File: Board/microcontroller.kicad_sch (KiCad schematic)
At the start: 31 parts, among them J10 FAN, J11 DUO LED, J9 ICSP, Q7 IRLML2502, SW1 CALIBRATE, U2 PIC18F2480-ISO, Y1 10 MHz

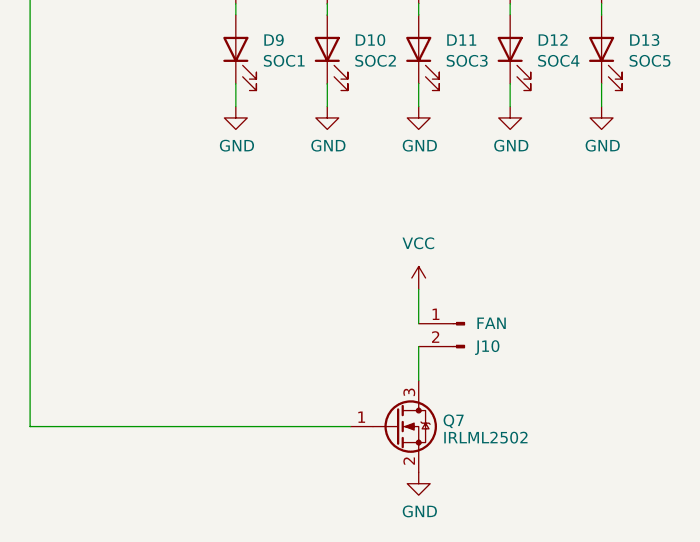
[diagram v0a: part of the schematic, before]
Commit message: New layout
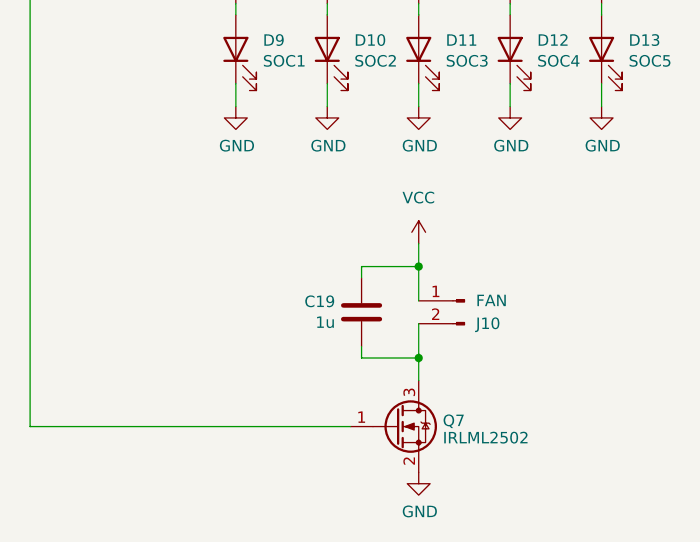
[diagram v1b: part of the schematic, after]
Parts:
- added C19: 1u, Capacitor_SMD:C_1206_3216Metric, symbol Device:C
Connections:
- net VCC: now also C19.1
- net at J10.2 (Pin_2), Q7.3 (D): now also C19.2
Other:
- moved on the sheet: J10
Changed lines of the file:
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@@
 	)
 	(junction
+		(at 231.14 142.24)
+		(diameter 0)
+		(color 0 0 0 0)
+	)
+	(junction
 		(at 217.17 57.15)
 		(diameter 0)
@@
 	)
 	(junction
+		(at 231.14 132.08)
+		(diameter 0)
+		(color 0 0 0 0)
+	)
+	(junction
 		(at 118.11 48.26)
 		(diameter 0)
@@
 	(wire
 		(pts
-			(xy 231.14 140.97) (xy 231.14 144.78)
+			(xy 231.14 138.43) (xy 231.14 142.24)
 		)
 		(stroke
@@
 	(wire
 		(pts
-			(xy 231.14 134.62) (xy 231.14 138.43)
+			(xy 231.14 129.54) (xy 231.14 132.08)
 		)
 		(stroke
@@
 	(wire
 		(pts
+			(xy 224.79 142.24) (xy 231.14 142.24)
+		)
+		(stroke
+			(width 0)
+			(type default)
+		)
+	)
+	(wire
+		(pts
 			(xy 168.91 120.65) (xy 149.86 120.65)
 		)
@@
 	(wire
 		(pts
+			(xy 224.79 133.35) (xy 224.79 132.08)
+		)
+		(stroke
+			(width 0)
+			(type default)
+		)
+	)
+	(wire
+		(pts
 			(xy 217.17 57.15) (xy 217.17 76.2)
 		)
@@
 	(wire
 		(pts
+			(xy 231.14 132.08) (xy 231.14 135.89)
+		)
+		(stroke
+			(width 0)
+			(type default)
+		)
+	)
+	(wire
+		(pts
 			(xy 220.98 114.3) (xy 220.98 111.76)
 		)
@@
 	(wire
 		(pts
+			(xy 224.79 132.08) (xy 231.14 132.08)
+		)
+		(stroke
+			(width 0)
+			(type default)
+		)
+	)
+	(wire
+		(pts
 			(xy 31.75 54.61) (xy 34.29 54.61)
 		)
@@
 	(wire
 		(pts
+			(xy 224.79 140.97) (xy 224.79 142.24)
+		)
+		(stroke
+			(width 0)
+			(type default)
+		)
+	)
+	(wire
+		(pts
 			(xy 148.59 73.66) (xy 201.93 73.66)
 		)
@@
 	(wire
 		(pts
+			(xy 231.14 142.24) (xy 231.14 144.78)
+		)
+		(stroke
+			(width 0)
+			(type default)
+		)
+	)
+	(wire
+		(pts
 			(xy 36.83 50.8) (xy 36.83 52.07)
 		)
@@
 	)
 	(symbol
+		(lib_id "Device:C")
+		(at 224.79 137.16 0)
+		(mirror y)
+		(unit 1)
+		(exclude_from_sim no)
+		(in_bom yes)
+		(on_board yes)
+		(dnp no)
+		(property "Reference" "C19"
+			(at 221.869 135.9916 0)
+			(effects
+				(font
+					(size 1.27 1.27)
+				)
+				(justify left)
+			)
+		)
+		(property "Value" "1u"
+			(at 221.869 138.303 0)
+			(effects
+				(font
+					(size 1.27 1.27)
+				)
+				(justify left)
+			)
+		)
+		(property "Footprint" "Capacitor_SMD:C_1206_3216Metric"
+			(at 223.8248 140.97 0)
+			(effects
+				(font
+					(size 1.27 1.27)
+				)
+				(hide yes)
+			)
+		)
+		(property "Datasheet" "~"
+			(at 224.79 137.16 0)
+			(effects
+				(font
+					(size 1.27 1.27)
+				)
+				(hide yes)
+			)
+		)
+		(property "Description" ""
+			(at 224.79 137.16 0)
+			(effects
+				(font
+					(size 1.27 1.27)
+				)
+				(hide yes)
+			)
+		)
+		(pin "1"
+		)
+		(pin "2"
+		)
+		(instances
+			(project "12VSupport"
+				(path "/f0c44745-560b-4dea-806a-2541c74a511b/3945f109-57ed-41f6-8253-6d6ba9eb298d"
+					(reference "C19")
+					(unit 1)
+				)
+			)
+		)
+	)
+	(symbol
 		(lib_id "power:GND")
 		(at 41.91 101.6 0)
@@
 	(symbol
 		(lib_id "Connector:Conn_01x02_Pin")
-		(at 236.22 138.43 0)
+		(at 236.22 135.89 0)
 		(mirror y)
 		(unit 1)
@@
 		(dnp no)
 		(property "Reference" "J10"
-			(at 237.49 140.9701 0)
+			(at 237.49 138.4301 0)
 			(effects
 				(font
@@
 		)
 		(property "Value" "FAN"
-			(at 237.49 138.4301 0)
+			(at 237.49 135.8901 0)
 			(effects
 				(font
@@
 		)
 		(property "Footprint" "Connector_JST:JST_XH_B2B-XH-A_1x02_P2.50mm_Vertical"
-			(at 236.22 138.43 0)
+			(at 236.22 135.89 0)
 			(effects
 				(font
@@
 		)
 		(property "Datasheet" "~"
-			(at 236.22 138.43 0)
+			(at 236.22 135.89 0)
 			(effects
 				(font
@@
 		)
 		(property "Description" "Generic connector, single row, 01x02, script generated"
-			(at 236.22 138.43 0)
+			(at 236.22 135.89 0)
 			(effects
 				(font
@@
 	(symbol
 		(lib_id "power:VCC")
-		(at 231.14 134.62 0)
+		(at 231.14 129.54 0)
 		(unit 1)
 		(exclude_from_sim no)
@@
 		(fields_autoplaced yes)
 		(property "Reference" "#PWR040"
-			(at 231.14 138.43 0)
+			(at 231.14 133.35 0)
 			(effects
 				(font
@@
 		)
 		(property "Value" "VCC"
-			(at 231.14 129.54 0)
+			(at 231.14 124.46 0)
 			(effects
 				(font
@@
 		)
 		(property "Footprint" ""
-			(at 231.14 134.62 0)
+			(at 231.14 129.54 0)
 			(effects
 				(font
@@
 		)
 		(property "Datasheet" ""
-			(at 231.14 134.62 0)
+			(at 231.14 129.54 0)
 			(effects
 				(font
@@
 		)
 		(property "Description" "Power symbol creates a global label with name \"VCC\""
-			(at 231.14 134.62 0)
+			(at 231.14 129.54 0)
 			(effects
 				(font
